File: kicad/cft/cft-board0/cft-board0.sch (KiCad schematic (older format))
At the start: 34 parts, among them P1 CFT-2021-Processor-Bus, P2 CFT-2021-Peripheral-Bus, U101 74LVC1G04, U102 74HC138, U103 74HC138, U104 74HC138, U105 74LVC1G32

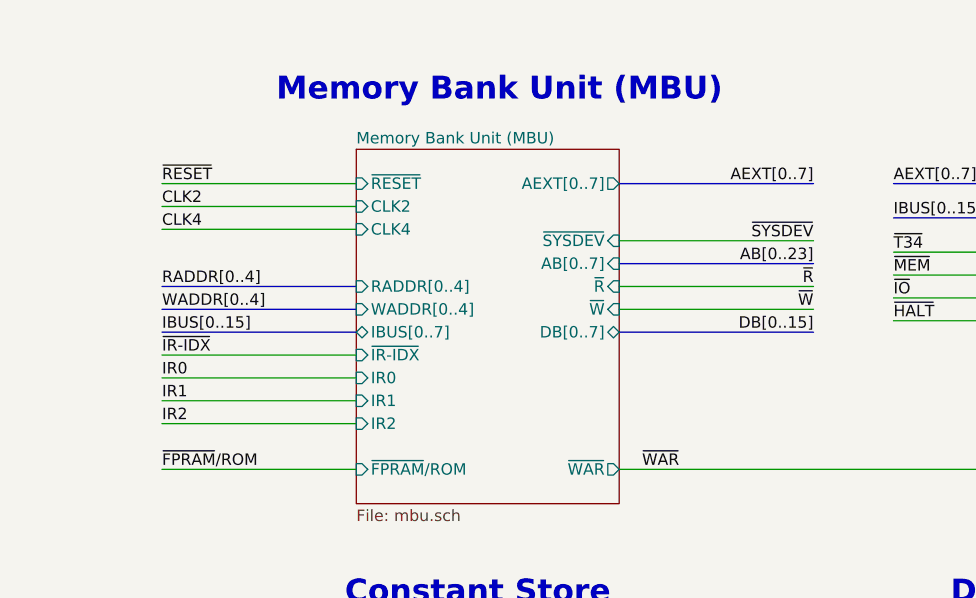
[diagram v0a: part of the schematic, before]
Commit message: Route MBU experimentally
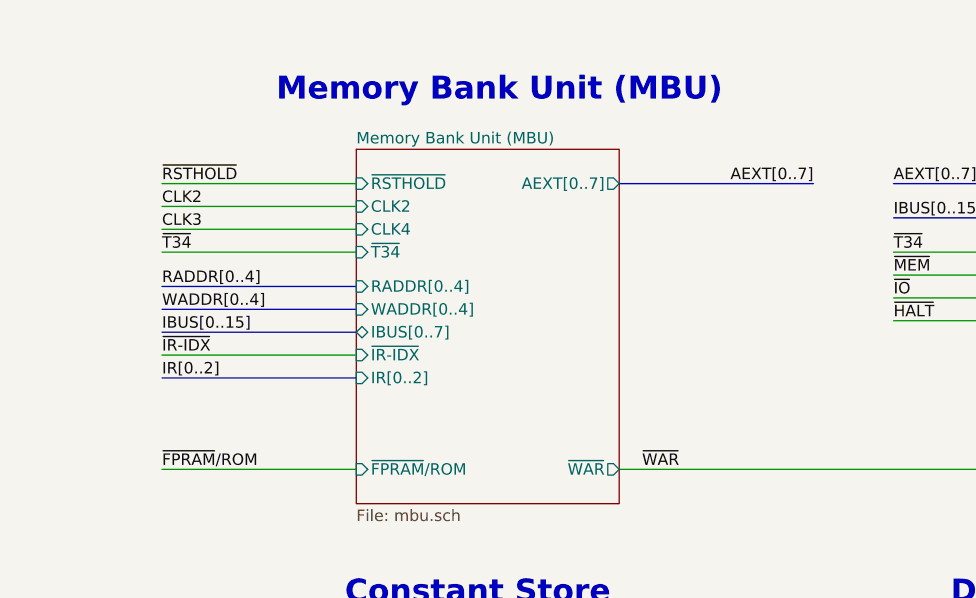
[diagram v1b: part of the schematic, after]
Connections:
- net labels added: IR[0..2]
- wire segments 431 -> 426
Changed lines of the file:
@@
 $Descr A4 11693 8268
 encoding utf-8
-Sheet 1 19
+Sheet 1 17
 Title "Control Unit Board"
 Date ""
@@
 ~FPAEXT
 Wire Wire Line
-	12150 -6450 13000 -6450
-Wire Wire Line
-	12150 -6150 13000 -6150
-Text Label 13000 -6450 2    50   ~ 0
-~SYSDEV
-Wire Bus Line
-	12150 -6350 13000 -6350
-Text Label 13000 -6350 2    50   ~ 0
-AB[0..23]
-Text Label 13000 -6150 2    50   ~ 0
-~W
-Wire Bus Line
-	12150 -6050 13000 -6050
-Text Label 13000 -6050 2    50   ~ 0
-DB[0..15]
-Wire Wire Line
 	11000 -5450 10150 -5450
 Text Label 10150 -5450 0    50   ~ 0
@@
 Wire Bus Line
 	11000 -6150 10150 -6150
-Text Label 10150 -6700 0    50   ~ 0
-~RESET
-Wire Wire Line
-	11000 -6700 10150 -6700
 Wire Wire Line
 	15350 -6200 16200 -6200
@@
 Address Register
 Wire Wire Line
-	11000 -5850 10150 -5850
-Wire Wire Line
-	11000 -5750 10150 -5750
-Text Label 10150 -5850 0    50   ~ 0
-IR0
-Text Label 10150 -5750 0    50   ~ 0
-IR1
-Wire Wire Line
-	12150 -6250 13000 -6250
-Text Label 13000 -6250 2    50   ~ 0
-~R
-Wire Wire Line
-	11000 -5650 10150 -5650
-Text Label 10150 -5650 0    50   ~ 0
-IR2
-Wire Wire Line
 	15300 -3650 16150 -3650
 Text Label 16150 -3650 2    50   ~ 0
@@
 Text Label 13350 -6100 0    50   ~ 0
 ~HALT
-Wire Wire Line
-	11000 -6600 10150 -6600
-Text Label 10150 -6600 0    50   ~ 0
-CLK2
-Wire Wire Line
-	11000 -6500 10150 -6500
-Text Label 10150 -6500 0    50   ~ 0
-CLK4
 $Sheet
 S 10950 -4650 1150 450
@@
 F0 "Memory Bank Unit (MBU)" 50
 F1 "mbu.sch" 50
-F2 "~RESET" I L 11000 -6700 50
-F3 "AEXT[0..7]" O R 12150 -6700 50
-F4 "WADDR[0..4]" I L 11000 -6150 50
-F5 "~FPRAM~∕ROM" I L 11000 -5450 50
-F6 "IBUS[0..7]" T L 11000 -6050 50
-F7 "RADDR[0..4]" I L 11000 -6250 50
-F8 "AB[0..7]" I R 12150 -6350 50
-F9 "~W" I R 12150 -6150 50
-F10 "~SYSDEV" I R 12150 -6450 50
-F11 "DB[0..7]" B R 12150 -6050 50
-F12 "~IR-IDX" I L 11000 -5950 50
-F13 "~WAR" O R 12150 -5450 50
-F14 "IR0" I L 11000 -5850 50
-F15 "IR1" I L 11000 -5750 50
-F16 "~R" I R 12150 -6250 50
-F17 "IR2" I L 11000 -5650 50
-F18 "CLK4" I L 11000 -6500 50
-F19 "CLK2" I L 11000 -6600 50
+F2 "AEXT[0..7]" O R 12150 -6700 50
+F3 "WADDR[0..4]" I L 11000 -6150 50
+F4 "~FPRAM~∕ROM" I L 11000 -5450 50
+F5 "IBUS[0..7]" T L 11000 -6050 50
+F6 "RADDR[0..4]" I L 11000 -6250 50
+F7 "~IR-IDX" I L 11000 -5950 50
+F8 "~WAR" O R 12150 -5450 50
+F9 "CLK4" I L 11000 -6500 50
+F10 "CLK2" I L 11000 -6600 50
+F11 "~RSTHOLD" I L 11000 -6700 50
+F12 "IR[0..2]" I L 11000 -5850 50
+F13 "~T34" I L 11000 -6400 50
 $EndSheet
 Wire Wire Line
@@
 $EndComp
 Wire Bus Line
+	11000 -5850 10150 -5850
+Text Label 10150 -5850 0    50   ~ 0
+IR[0..2]
+Wire Wire Line
+	11000 -6700 10150 -6700
+Wire Wire Line
+	11000 -6600 10150 -6600
+Wire Wire Line
+	11000 -6500 10150 -6500
+Wire Wire Line
+	11000 -6400 10150 -6400
+Wire Bus Line
 	2450 -4900 2450 -4100
 Wire Bus Line
@@
 Wire Bus Line
 	-10350 -3450 -10350 -2650
+Text Label 10150 -6700 0    50   ~ 0
+~RSTHOLD
+Text Label 10150 -6600 0    50   ~ 0
+CLK2
+Text Label 10150 -6500 0    50   ~ 0
+CLK3
+Text Label 10150 -6400 0    50   ~ 0
+~T34
 $EndSCHEMATC
